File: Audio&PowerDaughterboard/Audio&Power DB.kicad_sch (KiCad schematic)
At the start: 20 parts, among them J1 AudioJack3, J2 AudioJack3, J3 AudioJack3, J4 USB_C_Receptacle_USB2.0, J5 Conn_01x09, U1 SGTL5000XNLA3, U2 NCP1117-3.3_SOT223, U3 AP2127N-1.2

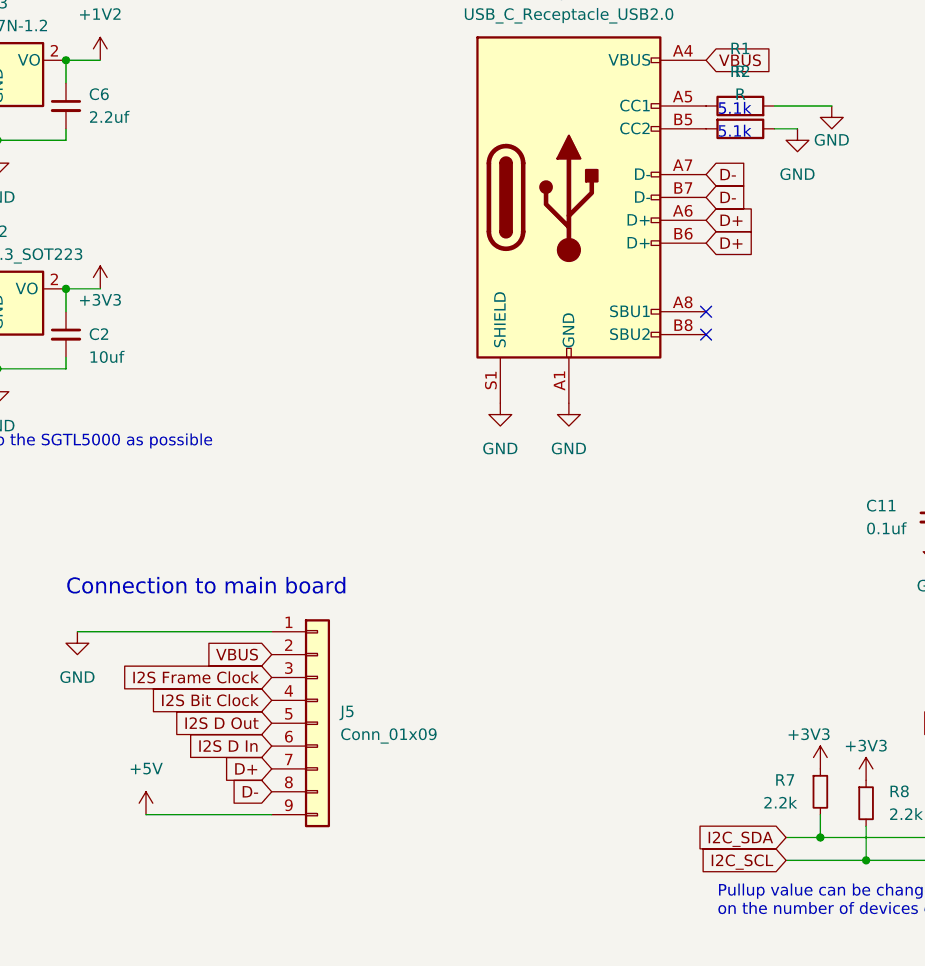
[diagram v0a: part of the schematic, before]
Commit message: Fuck this shi
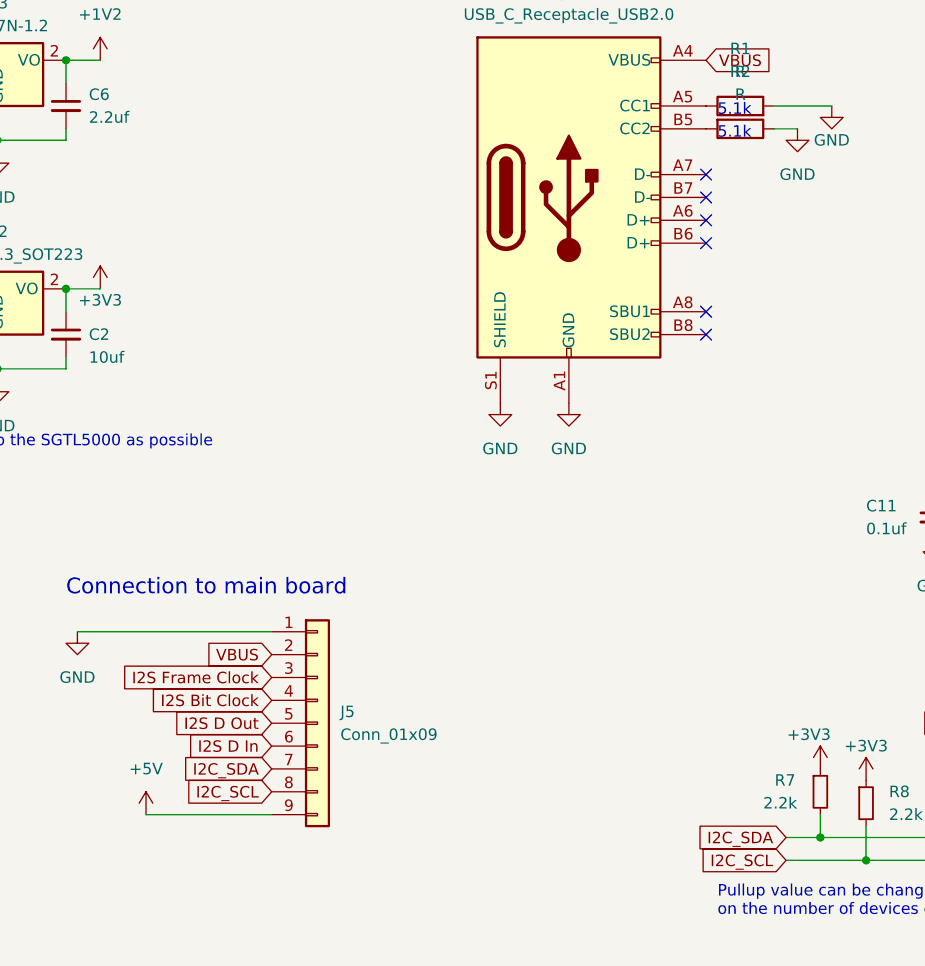
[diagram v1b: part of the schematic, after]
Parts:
- C1, C10, C11, C2, C6, C7, C8, C9: footprint (none) -> Capacitor_SMD:C_0603_1608Metric
- J1, J2, J3: footprint (none) -> Connector_Audio:Jack_3.5mm_CUI_SJ-3523-SMT_Horizontal
- J4: footprint (none) -> Connector_USB:USB_C_Receptacle_HRO_TYPE-C-31-M-12
- J5: footprint (none) -> Connector_JST:JST_SH_SM09B-SRSS-TB_1x09-1MP_P1.00mm_Horizontal
- R1, R2, R7, R8: footprint (none) -> Resistor_SMD:R_0603_1608Metric
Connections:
- net I2C_SCL: now also J5.8 (Pin_8)
- net I2C_SDA: now also J5.7 (Pin_7)
- removed net D+: J4.A6 (D+), J4.B6 (D+), J5.7 (Pin_7)
- removed net D-: J4.A7 (D-), J4.B7 (D-), J5.8 (Pin_8)
- no-connect marks 5 -> 9
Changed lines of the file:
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@@
   (no_connect (at 233.68 96.52))
   (no_connect (at 193.04 60.96))
+  (no_connect (at 193.04 53.34))
+  (no_connect (at 193.04 45.72))
+  (no_connect (at 193.04 50.8))
+  (no_connect (at 193.04 48.26))
   (no_connect (at 233.68 93.98))
   (no_connect (at 193.04 63.5))
@@
   (text "Connection to main board" (at 121.92 92.71 0)
     (effects (font (size 1.75 1.75)) (justify left bottom))
-  )
-  (global_label "D-" (shape input) (at 193.04 48.26 0) (fields_autoplaced)
-    (effects (font (size 1.27 1.27)) (justify left))
-    (property "Intersheetrefs" "${INTERSHEET_REFS}" (at 198.8676 48.26 0)
-      (effects (font (size 1.27 1.27)) (justify left) hide)
-    )
-  )
-  (global_label "D-" (shape input) (at 193.04 45.72 0) (fields_autoplaced)
-    (effects (font (size 1.27 1.27)) (justify left))
-    (property "Intersheetrefs" "${INTERSHEET_REFS}" (at 198.8676 45.72 0)
-      (effects (font (size 1.27 1.27)) (justify left) hide)
-    )
   )
   (global_label "I2C_SCL" (shape input) (at 201.93 121.92 180) (fields_autoplaced)
@@
     )
   )
-  (global_label "D+" (shape input) (at 144.78 111.76 180) (fields_autoplaced)
-    (effects (font (size 1.27 1.27)) (justify right))
-    (property "Intersheetrefs" "${INTERSHEET_REFS}" (at 138.9524 111.76 0)
-      (effects (font (size 1.27 1.27)) (justify right) hide)
-    )
-  )
   (global_label "I2S D Out" (shape input) (at 144.78 106.68 180) (fields_autoplaced)
     (effects (font (size 1.27 1.27)) (justify right))
     (property "Intersheetrefs" "${INTERSHEET_REFS}" (at 132.3606 106.68 0)
+      (effects (font (size 1.27 1.27)) (justify right) hide)
+    )
+  )
+  (global_label "I2C_SDA" (shape input) (at 144.78 111.76 180) (fields_autoplaced)
+    (effects (font (size 1.27 1.27)) (justify right))
+    (property "Intersheetrefs" "${INTERSHEET_REFS}" (at 134.1748 111.76 0)
       (effects (font (size 1.27 1.27)) (justify right) hide)
     )
@@
     )
   )
+  (global_label "I2C_SCL" (shape input) (at 144.78 114.3 180) (fields_autoplaced)
+    (effects (font (size 1.27 1.27)) (justify right))
+    (property "Intersheetrefs" "${INTERSHEET_REFS}" (at 134.2353 114.3 0)
+      (effects (font (size 1.27 1.27)) (justify right) hide)
+    )
+  )
   (global_label "Line In L" (shape input) (at 233.68 88.9 180) (fields_autoplaced)
     (effects (font (size 1.27 1.27)) (justify right))
@@
     )
   )
-  (global_label "D+" (shape input) (at 193.04 50.8 0) (fields_autoplaced)
-    (effects (font (size 1.27 1.27)) (justify left))
-    (property "Intersheetrefs" "${INTERSHEET_REFS}" (at 198.8676 50.8 0)
-      (effects (font (size 1.27 1.27)) (justify left) hide)
-    )
-  )
-  (global_label "D-" (shape input) (at 144.78 114.3 180) (fields_autoplaced)
-    (effects (font (size 1.27 1.27)) (justify right))
-    (property "Intersheetrefs" "${INTERSHEET_REFS}" (at 138.9524 114.3 0)
-      (effects (font (size 1.27 1.27)) (justify right) hide)
-    )
-  )
   (global_label "I2S Bit Clock" (shape input) (at 233.68 109.22 180) (fields_autoplaced)
     (effects (font (size 1.27 1.27)) (justify right))
@@
     )
   )
-  (global_label "D+" (shape input) (at 193.04 53.34 0) (fields_autoplaced)
-    (effects (font (size 1.27 1.27)) (justify left))
-    (property "Intersheetrefs" "${INTERSHEET_REFS}" (at 198.8676 53.34 0)
-      (effects (font (size 1.27 1.27)) (justify left) hide)
-    )
-  )
   (global_label "Line Out L" (shape input) (at 264.16 88.9 0) (fields_autoplaced)
     (effects (font (size 1.27 1.27)) (justify left))
@@
       (effects (font (size 1.27 1.27)) (justify left))
     )
-    (property "Footprint" "" (at 106.68 63.5 0)
+    (property "Footprint" "Capacitor_SMD:C_0603_1608Metric" (at 106.68 63.5 0)
       (effects (font (size 1.27 1.27)) hide)
     )
@@
       (effects (font (size 1.27 1.27)) (justify left))
     )
-    (property "Footprint" "" (at 210.82 115.57 0)
+    (property "Footprint" "Resistor_SMD:R_0603_1608Metric" (at 210.82 115.57 0)
       (effects (font (size 1.27 1.27)) hide)
     )
@@
       (effects (font (size 1.27 1.27)) (justify left))
     )
-    (property "Footprint" "" (at 121.92 38.1 0)
+    (property "Footprint" "Capacitor_SMD:C_0603_1608Metric" (at 121.92 38.1 0)
       (effects (font (size 1.27 1.27)) hide)
     )
@@
       (effects (font (size 1.27 1.27)) (justify left))
     )
-    (property "Footprint" "" (at 236.22 68.58 0)
+    (property "Footprint" "Capacitor_SMD:C_0603_1608Metric" (at 236.22 68.58 0)
       (effects (font (size 1.27 1.27)) hide)
     )
@@
       (effects (font (size 1.27 1.27)))
     )
-    (property "Footprint" "" (at 196.85 39.878 90)
+    (property "Footprint" "Resistor_SMD:R_0603_1608Metric" (at 196.85 39.878 90)
       (effects (font (size 1.27 1.27)) hide)
     )
@@
       (effects (font (size 1.27 1.27)) (justify left))
     )
-    (property "Footprint" "" (at 205.74 114.3 0)
+    (property "Footprint" "Resistor_SMD:R_0603_1608Metric" (at 205.74 114.3 0)
       (effects (font (size 1.27 1.27)) hide)
     )
@@
       (effects (font (size 1.27 1.27)))
     )
-    (property "Footprint" "" (at 181.61 48.26 0)
+    (property "Footprint" "Connector_USB:USB_C_Receptacle_HRO_TYPE-C-31-M-12" (at 181.61 48.26 0)
       (effects (font (size 1.27 1.27)) hide)
     )
@@
       (effects (font (size 1.27 1.27)))
     )
-    (property "Footprint" "" (at 45.72 73.66 0)
+    (property "Footprint" "Connector_Audio:Jack_3.5mm_CUI_SJ-3523-SMT_Horizontal" (at 45.72 73.66 0)
       (effects (font (size 1.27 1.27)) hide)
     )
@@
       (effects (font (size 1.27 1.27)))
     )
-    (property "Footprint" "" (at 45.72 48.26 0)
+    (property "Footprint" "Connector_Audio:Jack_3.5mm_CUI_SJ-3523-SMT_Horizontal" (at 45.72 48.26 0)
       (effects (font (size 1.27 1.27)) hide)
     )
@@
       (effects (font (size 1.27 1.27)))
     )
-    (property "Footprint" "" (at 45.72 99.06 0)
+    (property "Footprint" "Connector_Audio:Jack_3.5mm_CUI_SJ-3523-SMT_Horizontal" (at 45.72 99.06 0)
       (effects (font (size 1.27 1.27)) hide)
     )
@@
       (effects (font (size 1.27 1.27)) (justify left))
     )
-    (property "Footprint" "" (at 243.84 55.88 0)
+    (property "Footprint" "Capacitor_SMD:C_0603_1608Metric" (at 243.84 55.88 0)
       (effects (font (size 1.27 1.27)) hide)
     )
@@
       (effects (font (size 1.27 1.27)) (justify left))
     )
-    (property "Footprint" "" (at 232.41 68.58 0)
+    (property "Footprint" "Capacitor_SMD:C_0603_1608Metric" (at 232.41 68.58 0)
       (effects (font (size 1.27 1.27)) hide)
     )
@@
       (effects (font (size 1.27 1.27)) (justify left))
     )
-    (property "Footprint" "" (at 121.92 63.5 0)
+    (property "Footprint" "Capacitor_SMD:C_0603_1608Metric" (at 121.92 63.5 0)
       (effects (font (size 1.27 1.27)) hide)
     )
@@
       (effects (font (size 1.27 1.27)) (justify left))
     )
-    (property "Footprint" "" (at 218.44 83.82 0)
+    (property "Footprint" "Capacitor_SMD:C_0603_1608Metric" (at 218.44 83.82 0)
       (effects (font (size 1.27 1.27)) hide)
     )
@@
       (effects (font (size 1.27 1.27)))
     )
-    (property "Footprint" "" (at 196.85 38.862 90)
+    (property "Footprint" "Resistor_SMD:R_0603_1608Metric" (at 196.85 38.862 90)
       (effects (font (size 1.27 1.27)) hide)
     )
@@
       (effects (font (size 1.27 1.27)) (justify left))
     )
-    (property "Footprint" "" (at 149.86 106.68 0)
+    (property "Footprint" "Connector_JST:JST_SH_SM09B-SRSS-TB_1x09-1MP_P1.00mm_Horizontal" (at 149.86 106.68 0)
       (effects (font (size 1.27 1.27)) hide)
     )
@@
       (effects (font (size 1.27 1.27)) (justify left))
     )
-    (property "Footprint" "" (at 106.68 38.1 0)
-      (effects (font (size 1.27 1.27)) hide)
-    )
+    (property "Footprint" "Capacitor_SMD:C_0603_1608Metric" (at 106.68 38.1 0)
+      (effects (font (size 1.27 1.27)) hide)
+    )

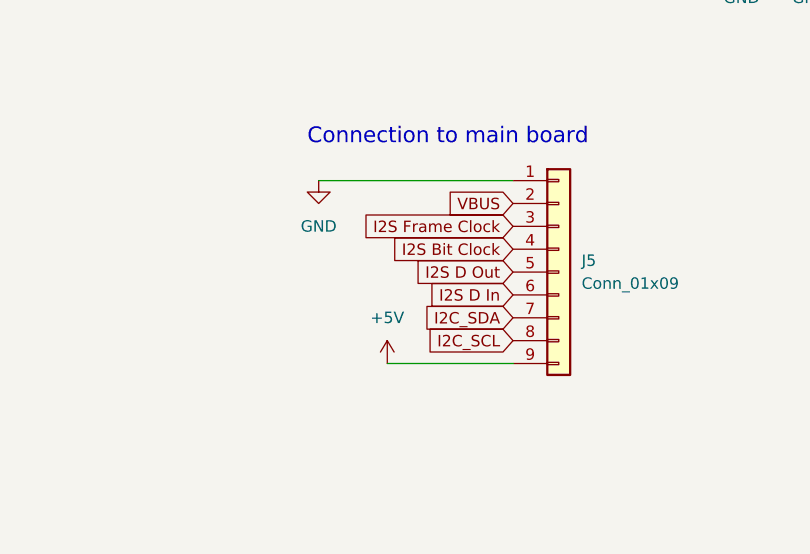
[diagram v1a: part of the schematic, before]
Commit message: FIN
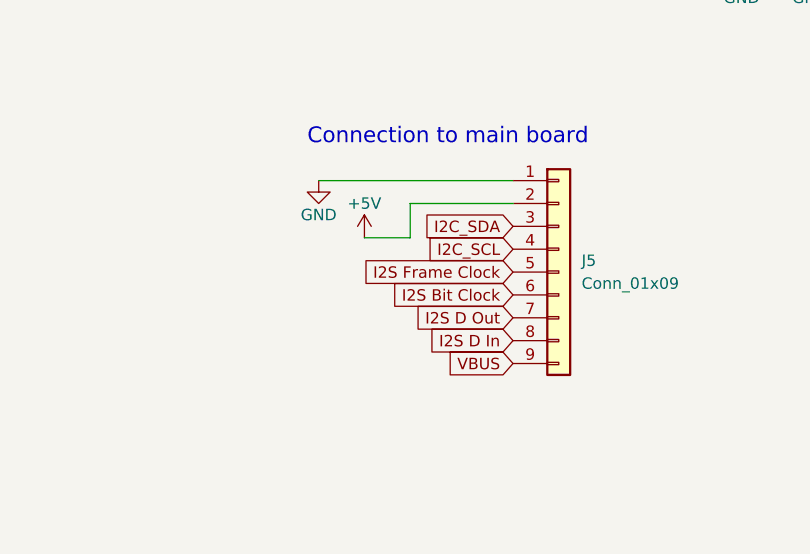
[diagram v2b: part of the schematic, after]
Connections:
- net +5V: now also J5.2 (Pin_2); no longer J5.9 (Pin_9)
- net I2C_SCL: now also J5.4 (Pin_4); no longer J5.8 (Pin_8)
- net I2C_SDA: now also J5.3 (Pin_3); no longer J5.7 (Pin_7)
- net I2S Bit Clock: now also J5.6 (Pin_6); no longer J5.4 (Pin_4)
- net I2S D In: now also J5.8 (Pin_8); no longer J5.6 (Pin_6)
- net I2S D Out: now also J5.7 (Pin_7); no longer J5.5 (Pin_5)
- net I2S Frame Clock: now also J5.5 (Pin_5); no longer J5.3 (Pin_3)
- net VBUS: now also J5.9 (Pin_9); no longer J5.2 (Pin_2)
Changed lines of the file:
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@@
-    (stroke (width 0) (type default))
-  )
-  (wire (pts (xy 130.81 116.84) (xy 144.78 116.84))
     (stroke (width 0) (type default))
   )
@@
     (stroke (width 0) (type default))
   )
+  (wire (pts (xy 133.35 99.06) (xy 144.78 99.06))
+    (stroke (width 0) (type default))
+  )
   (wire (pts (xy 114.3 41.91) (xy 114.3 43.18))
     (stroke (width 0) (type default))
   )
+  (wire (pts (xy 133.35 102.87) (xy 133.35 99.06))
+    (stroke (width 0) (type default))
+  )
   (wire (pts (xy 106.68 40.64) (xy 106.68 41.91))
     (stroke (width 0) (type default))
@@
   )
   (wire (pts (xy 121.92 66.04) (xy 121.92 67.31))
+    (stroke (width 0) (type default))
+  )
+  (wire (pts (xy 128.27 102.87) (xy 133.35 102.87))
     (stroke (width 0) (type default))
   )
@@
     (effects (font (size 1.75 1.75)) (justify left bottom))
   )
+  (global_label "I2C_SCL" (shape input) (at 144.78 104.14 180) (fields_autoplaced)
+    (effects (font (size 1.27 1.27)) (justify right))
+    (property "Intersheetrefs" "${INTERSHEET_REFS}" (at 134.2353 104.14 0)
+      (effects (font (size 1.27 1.27)) (justify right) hide)
+    )
+  )
   (global_label "I2C_SCL" (shape input) (at 201.93 121.92 180) (fields_autoplaced)
     (effects (font (size 1.27 1.27)) (justify right))
@@
     )
   )
-  (global_label "I2S Bit Clock" (shape input) (at 144.78 104.14 180) (fields_autoplaced)
-    (effects (font (size 1.27 1.27)) (justify right))
-    (property "Intersheetrefs" "${INTERSHEET_REFS}" (at 129.0344 104.14 0)
+  (global_label "I2S Frame Clock" (shape input) (at 144.78 106.68 180) (fields_autoplaced)
+    (effects (font (size 1.27 1.27)) (justify right))
+    (property "Intersheetrefs" "${INTERSHEET_REFS}" (at 125.8292 106.68 0)
       (effects (font (size 1.27 1.27)) (justify right) hide)
     )
@@
     )
   )
-  (global_label "I2S D Out" (shape input) (at 144.78 106.68 180) (fields_autoplaced)
-    (effects (font (size 1.27 1.27)) (justify right))
-    (property "Intersheetrefs" "${INTERSHEET_REFS}" (at 132.3606 106.68 0)
-      (effects (font (size 1.27 1.27)) (justify right) hide)
-    )
-  )
-  (global_label "I2C_SDA" (shape input) (at 144.78 111.76 180) (fields_autoplaced)
-    (effects (font (size 1.27 1.27)) (justify right))
-    (property "Intersheetrefs" "${INTERSHEET_REFS}" (at 134.1748 111.76 0)
-      (effects (font (size 1.27 1.27)) (justify right) hide)
-    )
-  )
-  (global_label "VBUS" (shape input) (at 144.78 99.06 180) (fields_autoplaced)
-    (effects (font (size 1.27 1.27)) (justify right))
-    (property "Intersheetrefs" "${INTERSHEET_REFS}" (at 136.8962 99.06 0)
+  (global_label "I2C_SDA" (shape input) (at 144.78 101.6 180) (fields_autoplaced)
+    (effects (font (size 1.27 1.27)) (justify right))
+    (property "Intersheetrefs" "${INTERSHEET_REFS}" (at 134.1748 101.6 0)
       (effects (font (size 1.27 1.27)) (justify right) hide)
     )
@@
     )
   )
-  (global_label "I2S D In" (shape input) (at 144.78 109.22 180) (fields_autoplaced)
-    (effects (font (size 1.27 1.27)) (justify right))
-    (property "Intersheetrefs" "${INTERSHEET_REFS}" (at 133.812 109.22 0)
-      (effects (font (size 1.27 1.27)) (justify right) hide)
-    )
-  )
-  (global_label "I2C_SCL" (shape input) (at 144.78 114.3 180) (fields_autoplaced)
-    (effects (font (size 1.27 1.27)) (justify right))
-    (property "Intersheetrefs" "${INTERSHEET_REFS}" (at 134.2353 114.3 0)
+  (global_label "I2S Bit Clock" (shape input) (at 144.78 109.22 180) (fields_autoplaced)
+    (effects (font (size 1.27 1.27)) (justify right))
+    (property "Intersheetrefs" "${INTERSHEET_REFS}" (at 129.0344 109.22 0)
       (effects (font (size 1.27 1.27)) (justify right) hide)
     )
@@
     )
   )
+  (global_label "I2S D Out" (shape input) (at 144.78 111.76 180) (fields_autoplaced)
+    (effects (font (size 1.27 1.27)) (justify right))
+    (property "Intersheetrefs" "${INTERSHEET_REFS}" (at 132.3606 111.76 0)
+      (effects (font (size 1.27 1.27)) (justify right) hide)
+    )
+  )
   (global_label "HP_L" (shape input) (at 264.16 109.22 0) (fields_autoplaced)
     (effects (font (size 1.27 1.27)) (justify left))
@@
     )
   )
+  (global_label "VBUS" (shape input) (at 144.78 116.84 180) (fields_autoplaced)
+    (effects (font (size 1.27 1.27)) (justify right))
+    (property "Intersheetrefs" "${INTERSHEET_REFS}" (at 136.8962 116.84 0)
+      (effects (font (size 1.27 1.27)) (justify right) hide)
+    )
+  )
   (global_label "Line Out L" (shape input) (at 264.16 88.9 0) (fields_autoplaced)
     (effects (font (size 1.27 1.27)) (justify left))
@@
     )
   )
-  (global_label "I2S Frame Clock" (shape input) (at 144.78 101.6 180) (fields_autoplaced)
-    (effects (font (size 1.27 1.27)) (justify right))
-    (property "Intersheetrefs" "${INTERSHEET_REFS}" (at 125.8292 101.6 0)
-      (effects (font (size 1.27 1.27)) (justify right) hide)
-    )
-  )
   (global_label "HP_VGND" (shape input) (at 264.16 106.68 0) (fields_autoplaced)
     (effects (font (size 1.27 1.27)) (justify left))
@@
     (property "Intersheetrefs" "${INTERSHEET_REFS}" (at 62.3728 76.2 0)
       (effects (font (size 1.27 1.27)) (justify left) hide)
+    )
+  )
+  (global_label "I2S D In" (shape input) (at 144.78 114.3 180) (fields_autoplaced)
+    (effects (font (size 1.27 1.27)) (justify right))
+    (property "Intersheetrefs" "${INTERSHEET_REFS}" (at 133.812 114.3 0)
+      (effects (font (size 1.27 1.27)) (justify right) hide)
     )
   )
@@
     )
   )
-  (symbol (lib_id "power:+5V") (at 130.81 116.84 0) (unit 1)
-    (in_bom yes) (on_board yes) (dnp no) (fields_autoplaced)
-    (property "Reference" "#PWR016" (at 130.81 120.65 0)
-      (effects (font (size 1.27 1.27)) hide)
-    )
-    (property "Value" "+5V" (at 130.81 111.76 0)
-      (effects (font (size 1.27 1.27)))
-    )
-    (property "Footprint" "" (at 130.81 116.84 0)
-      (effects (font (size 1.27 1.27)) hide)
-    )
-    (property "Datasheet" "" (at 130.81 116.84 0)
-      (effects (font (size 1.27 1.27)) hide)
-    )
-    (pin "1")
-    (instances
-      (project "Audio&Power DB"
-        (path "/efee3861-08c8-4ee5-870a-4ef6b30a8ea3"
-          (reference "#PWR016") (unit 1)
-        )
-      )
-    )
-  )
   (symbol (lib_id "power:GND") (at 243.84 58.42 0) (unit 1)
     (in_bom yes) (on_board yes) (dnp no)
@@
   )
   (symbol (lib_id "power:GND") (at 123.19 96.52 0) (unit 1)
-    (in_bom yes) (on_board yes) (dnp no) (fields_autoplaced)
+    (in_bom yes) (on_board yes) (dnp no)
     (property "Reference" "#PWR017" (at 123.19 102.87 0)
       (effects (font (size 1.27 1.27)) hide)
     )
-    (property "Value" "GND" (at 123.19 101.6 0)
+    (property "Value" "GND" (at 123.19 100.33 0)
       (effects (font (size 1.27 1.27)))
     )
@@
         )
       )
+    )
+  )
+  (symbol (lib_id "power:+5V") (at 128.27 102.87 0) (unit 1)
+    (in_bom yes) (on_board yes) (dnp no)
+    (property "Reference" "#PWR015" (at 128.27 106.68 0)
+      (effects (font (size 1.27 1.27)) hide)
+    )
+    (property "Value" "+5V" (at 128.27 99.06 0)
+      (effects (font (size 1.27 1.27)))
+    )
+    (property "Footprint" "" (at 128.27 102.87 0)
+      (effects (font (size 1.27 1.27)) hide)
+    )
+    (property "Datasheet" "" (at 128.27 102.87 0)
+      (effects (font (size 1.27 1.27)) hide)
+    )
+    (pin "1")
+    (instances
+      (project "Audio&Power DB"
+        (path "/efee3861-08c8-4ee5-870a-4ef6b30a8ea3"
+          (reference "#PWR015") (unit 1)
+        )
+      )
